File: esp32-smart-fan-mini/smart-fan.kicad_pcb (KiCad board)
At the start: 2 copper layers, 78.7 x 33 mm, 12 parts, among them J1 Screw_Terminal_01x02, J6 Screw_Terminal_01x02, M1 MP1584-Module, SW1 RotaryEncoder_Switch, U1 mini_esp32

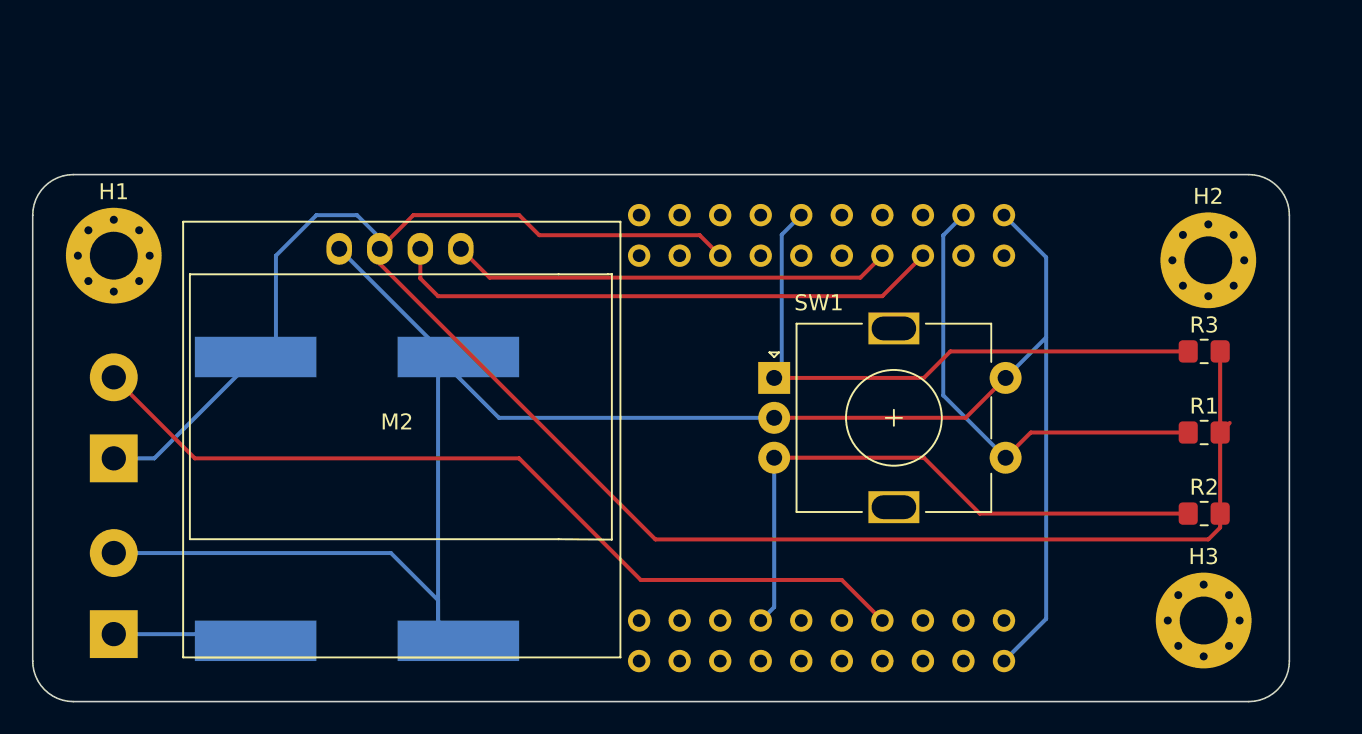
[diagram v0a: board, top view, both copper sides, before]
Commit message: Update panalize
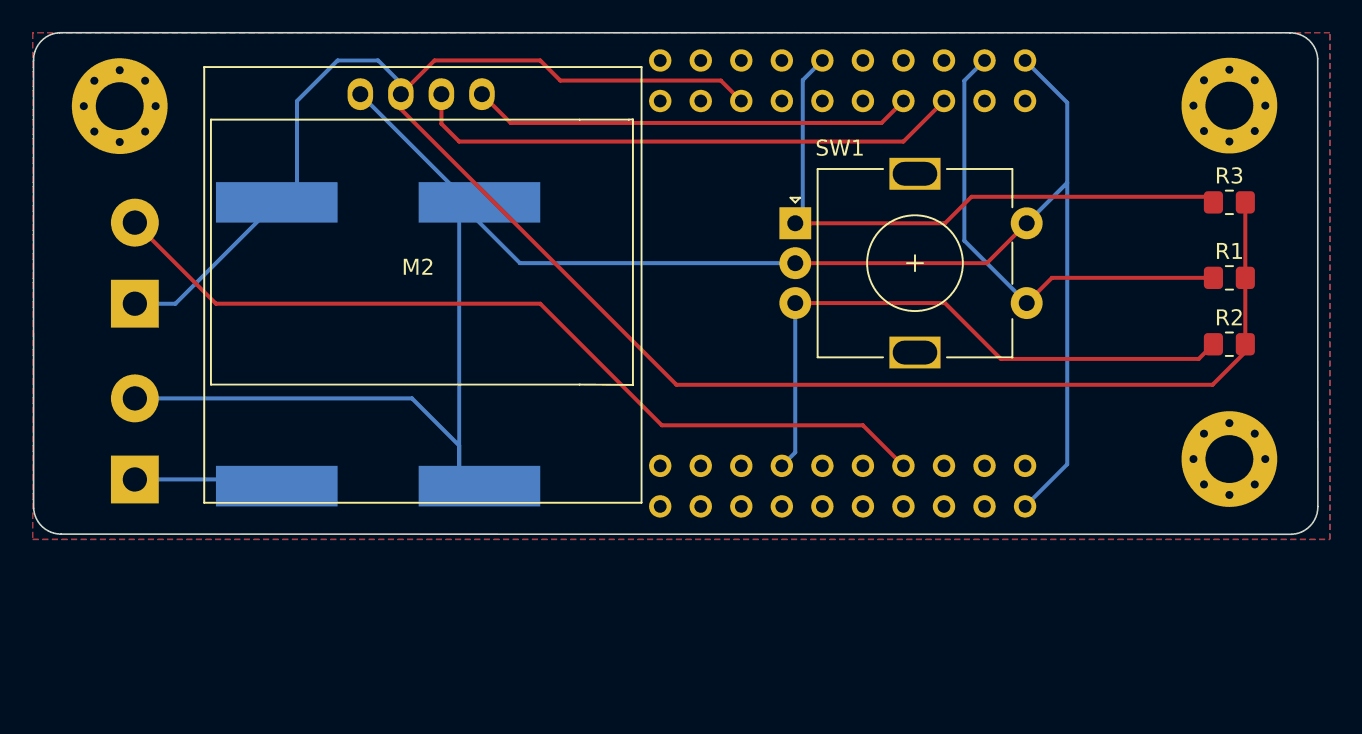
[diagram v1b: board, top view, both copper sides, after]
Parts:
- moved R2 10.7 mm to (125.8, 89.4)
- moved H3 10.2 mm to (125.8, 96.6)
- moved R1 9.82 mm to (125.8, 85.2)
- moved H2 9.78 mm to (125.8, 74.4)
- moved J6 9.78 mm to (57.2, 97.8)
- moved M1 9.78 mm to (72.4, 89.4)
- moved U1 9.78 mm to (101.5, 85.6)
- moved SW1 9.78 mm to (98.6, 81.8)
- moved J1 9.78 mm to (57.2, 86.8)
- moved M2 9.78 mm to (74.9, 84.3)
- moved R3 9.47 mm to (125.8, 80.5)
- moved H1 9.38 mm to (56.3, 74.5)
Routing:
- net 5V: track 126.7 -> 125.0 mm
- net IO5: track 37.9 -> 38.6 mm
- added copper zone on B.Cu, net GND
- added copper zone on F.Cu, net GND
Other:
- board size 78.7 x 33 mm -> 80.5 x 31.4 mm
